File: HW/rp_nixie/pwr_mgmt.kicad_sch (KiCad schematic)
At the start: 2 parts, among them U1 MC33063AD

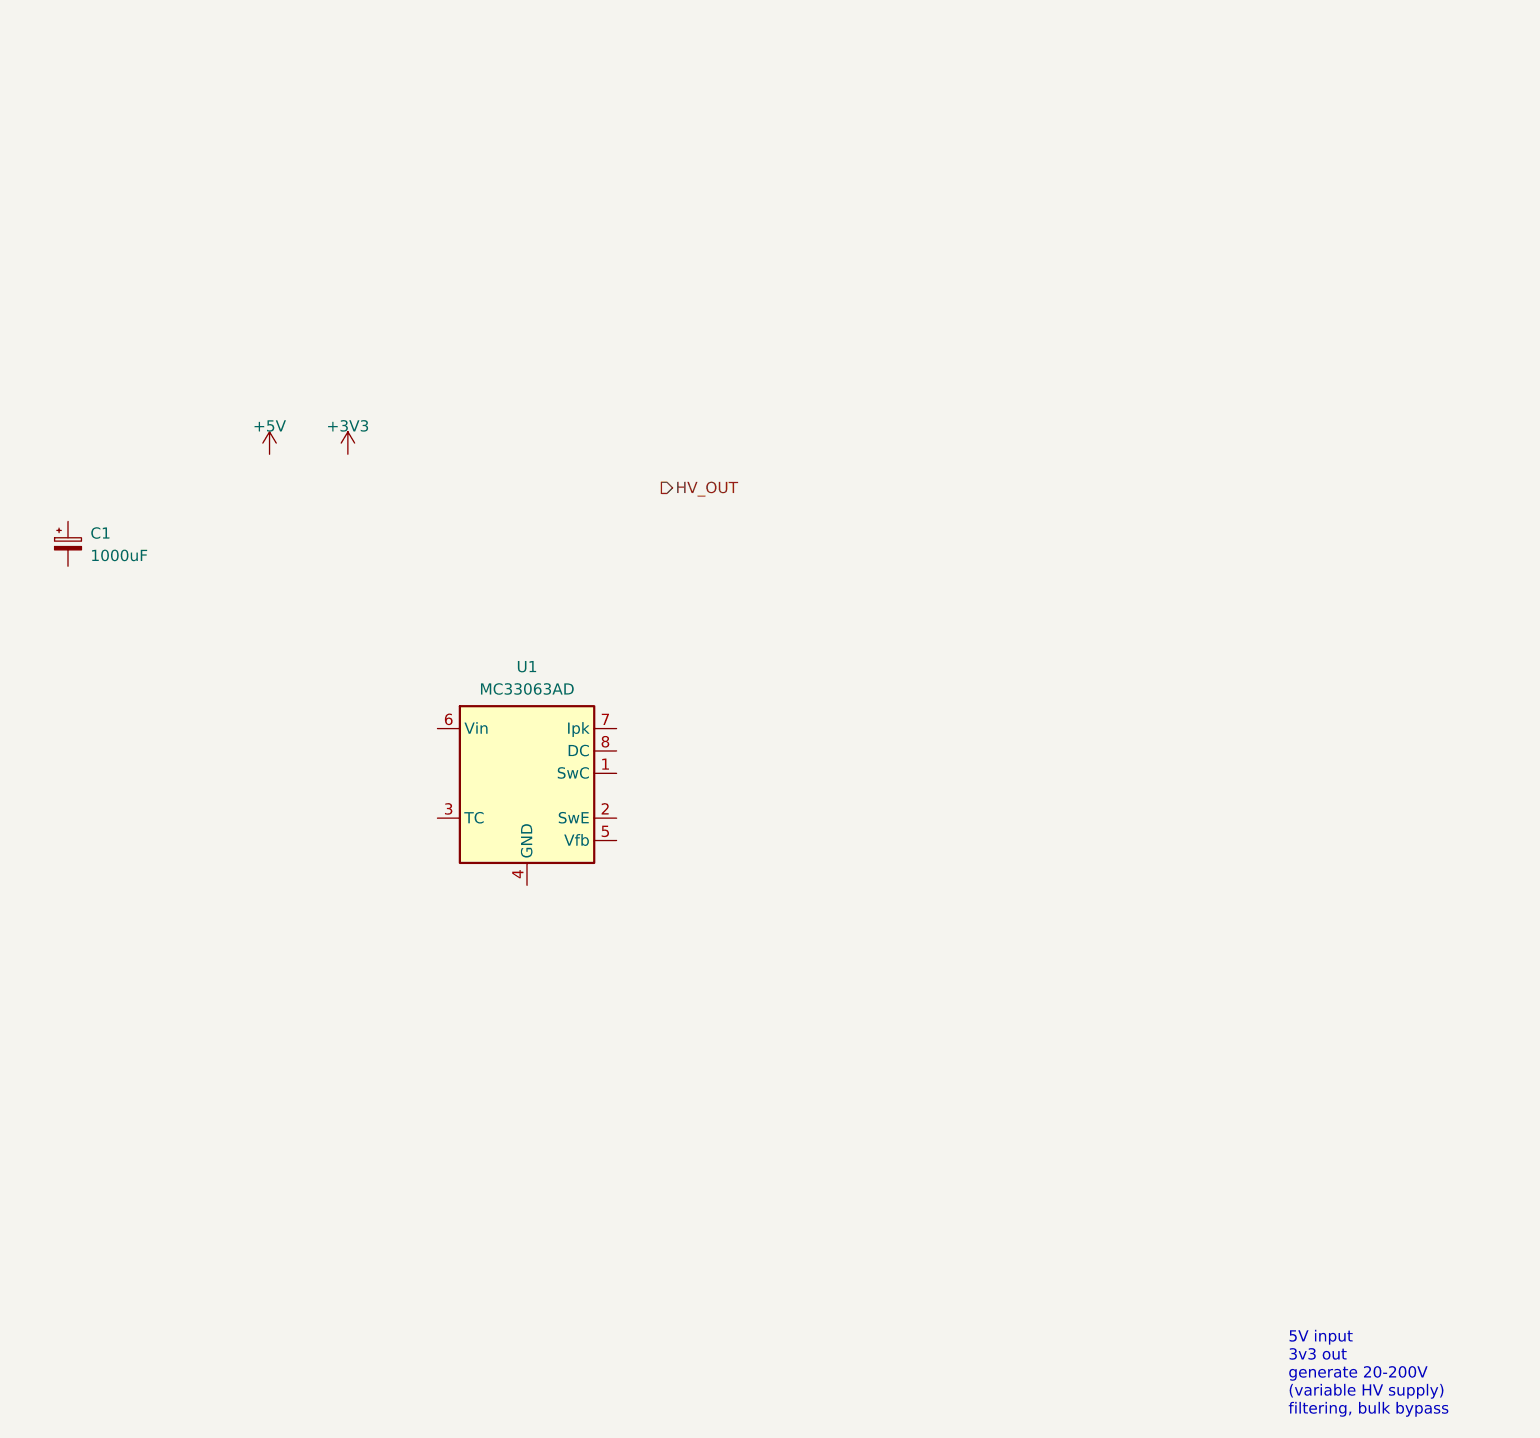
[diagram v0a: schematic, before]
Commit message: finished MCU and IO
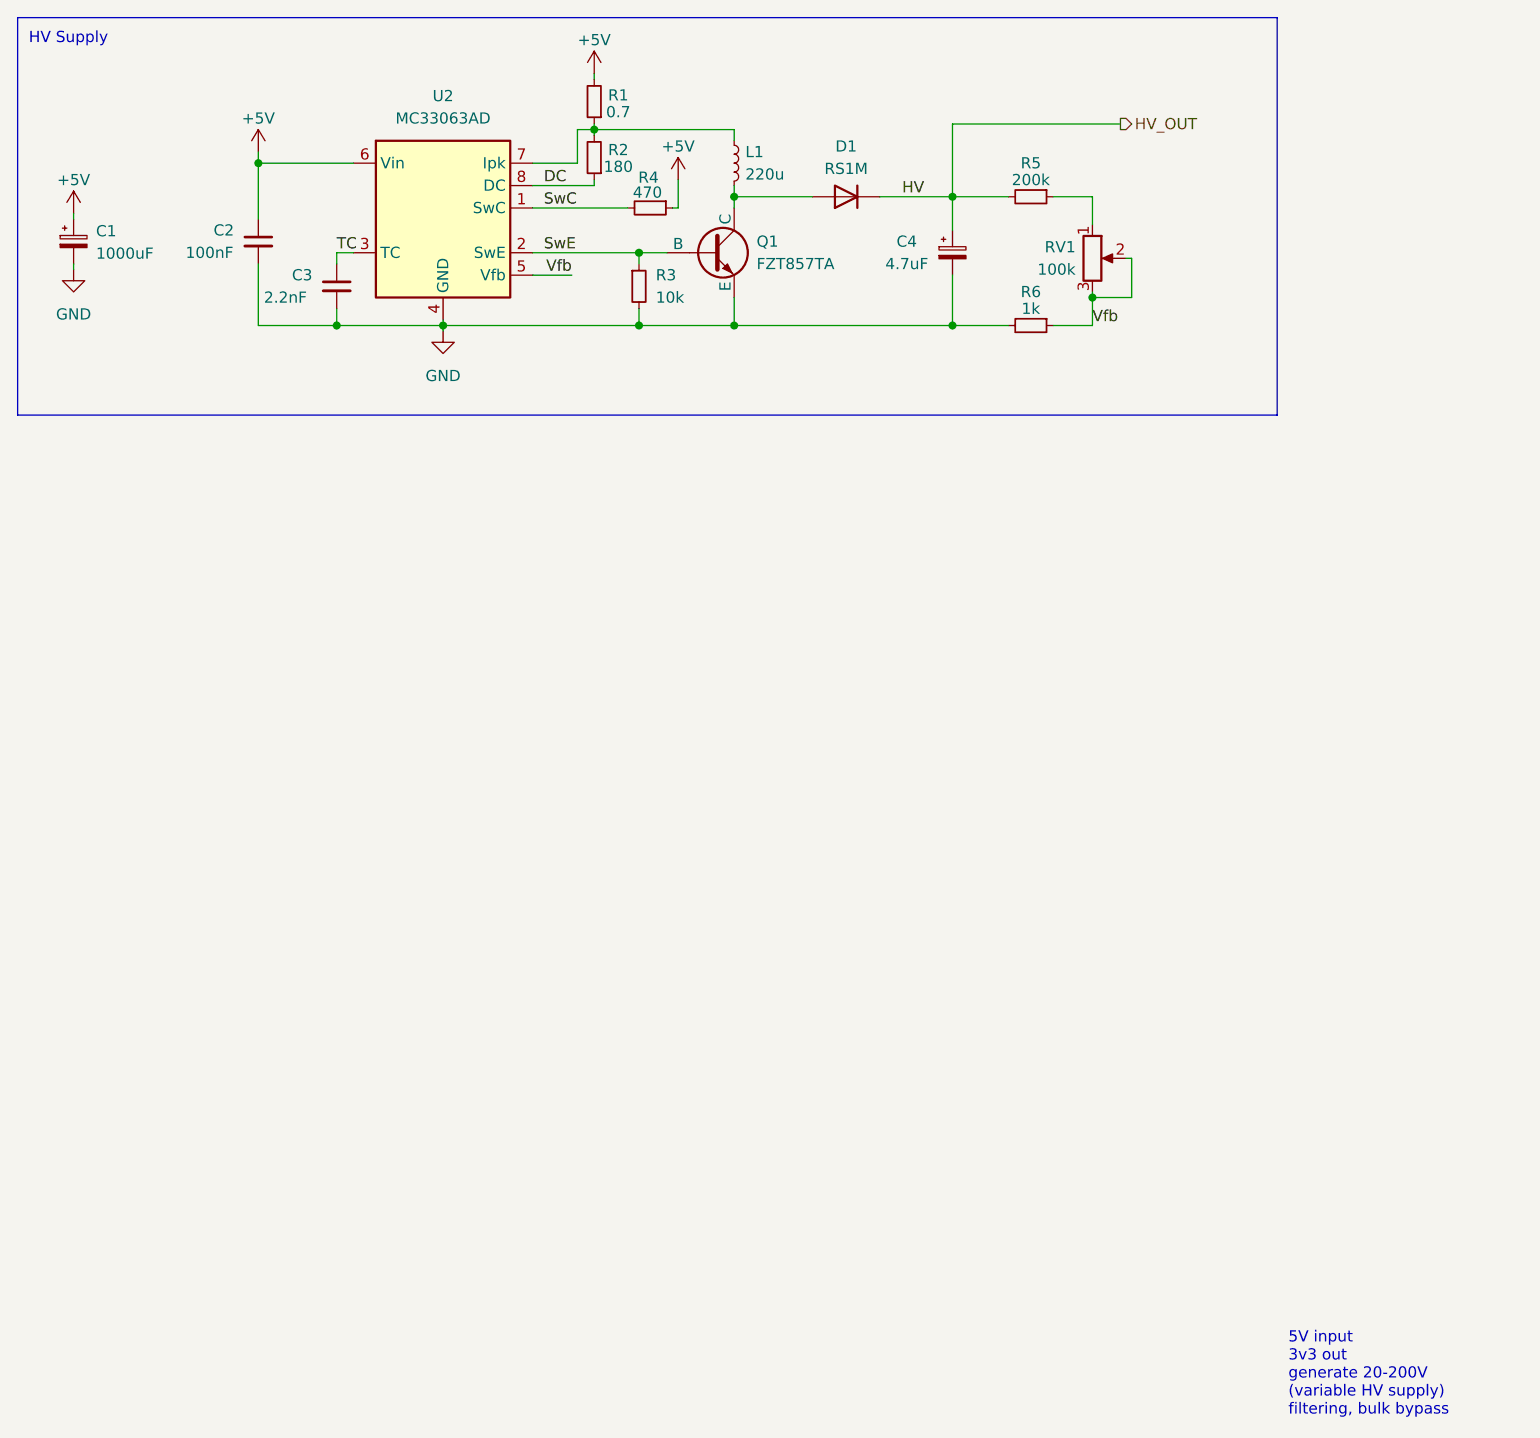
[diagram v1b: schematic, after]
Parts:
- removed U1: MC33063AD, Package_SO:SOIC-8_3.9x4.9mm_P1.27mm, symbol Regulator_Switching:MC33063AD
- added C2: 100nF, symbol Device:C_Small
- added C3: 2.2nF, symbol Device:C_Small
- added C4: 4.7uF, Capacitor_SMD:CP_Elec_10x10, symbol Device:C_Polarized_Small
- added D1: RS1M, symbol Device:D
- added L1: 220u, symbol Device:L_Small
- added Q1: FZT857TA, symbol Simulation_SPICE:NPN
- added R1: 0.7, symbol Device:R_Small
- added R2: 180, symbol Device:R_Small
- added R3: 10k, symbol Device:R_Small
- added R4: 470, symbol Device:R_Small
- added R5: 200k, symbol Device:R_Small
- added R6: 1k, symbol Device:R_Small
- added RV1: 100k, symbol Device:R_Potentiometer
- added U2: MC33063AD, Package_SO:SOIC-8_3.9x4.9mm_P1.27mm, symbol Regulator_Switching:MC33063AD
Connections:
- net +5V: now also C1.1, C2.1, R1.2, R4.1, U2.6 (Vin)
- net HV_OUT: now also C4.1, D1.1 (K), R5.2
- net GND: now reaches C1.2
- net GND: now also C2.2, C3.2, C4.2, Q1.3 (E), R3.2, R6.2, U2.4 (GND)
- new net: L1.1, R1.1, R2.2, U2.7 (Ipk)
- new net: D1.2 (A), L1.2, Q1.1 (C)
- new net: R5.1, RV1.1
- new net DC: R2.1, U2.8 (DC)
- new net SwC: R4.2, U2.1 (SwC)
- new net SwE: Q1.2 (B), R3.1, U2.2 (SwE)
- new net TC: C3.1, U2.3 (TC)
- new net Vfb: R6.1, RV1.2, RV1.3, U2.5 (Vfb)
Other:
- note added: "HV Supply"
- moved on the sheet: C1
